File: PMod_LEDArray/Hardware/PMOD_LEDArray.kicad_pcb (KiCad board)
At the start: 2 copper layers, 81.6 x 23 mm, 133 parts, among them J1 Conn_02x06_Odd_Even, U1 GN1640

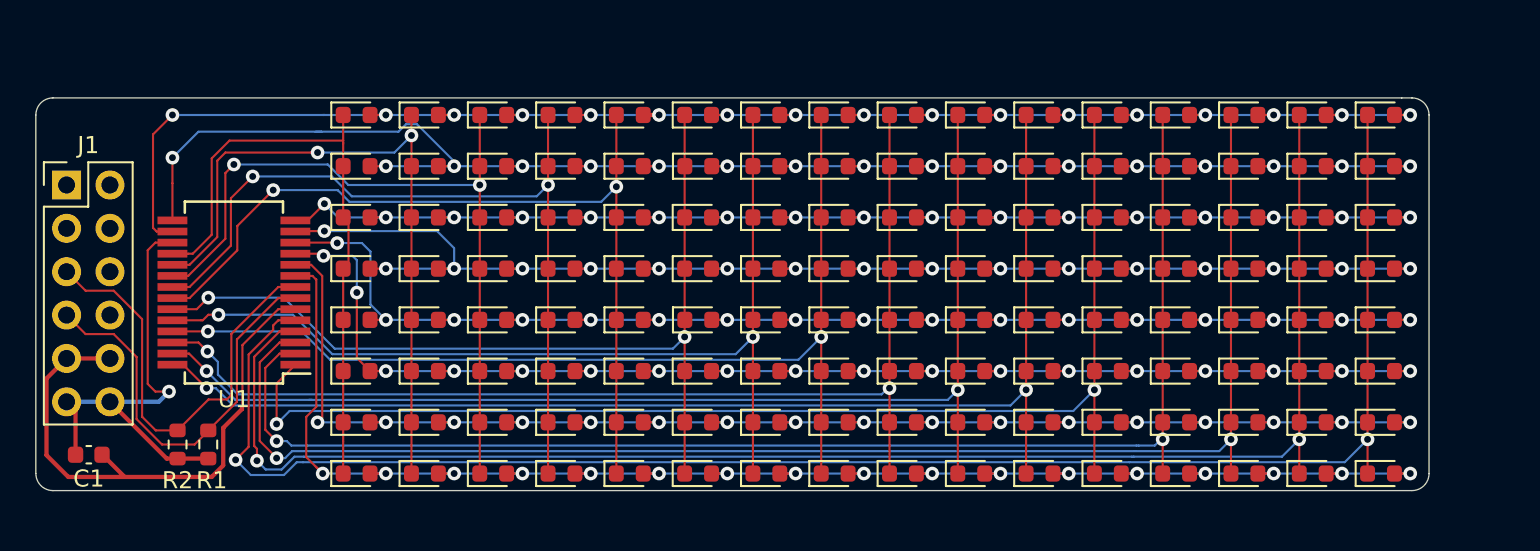
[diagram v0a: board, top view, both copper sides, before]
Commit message: Add mounting holes
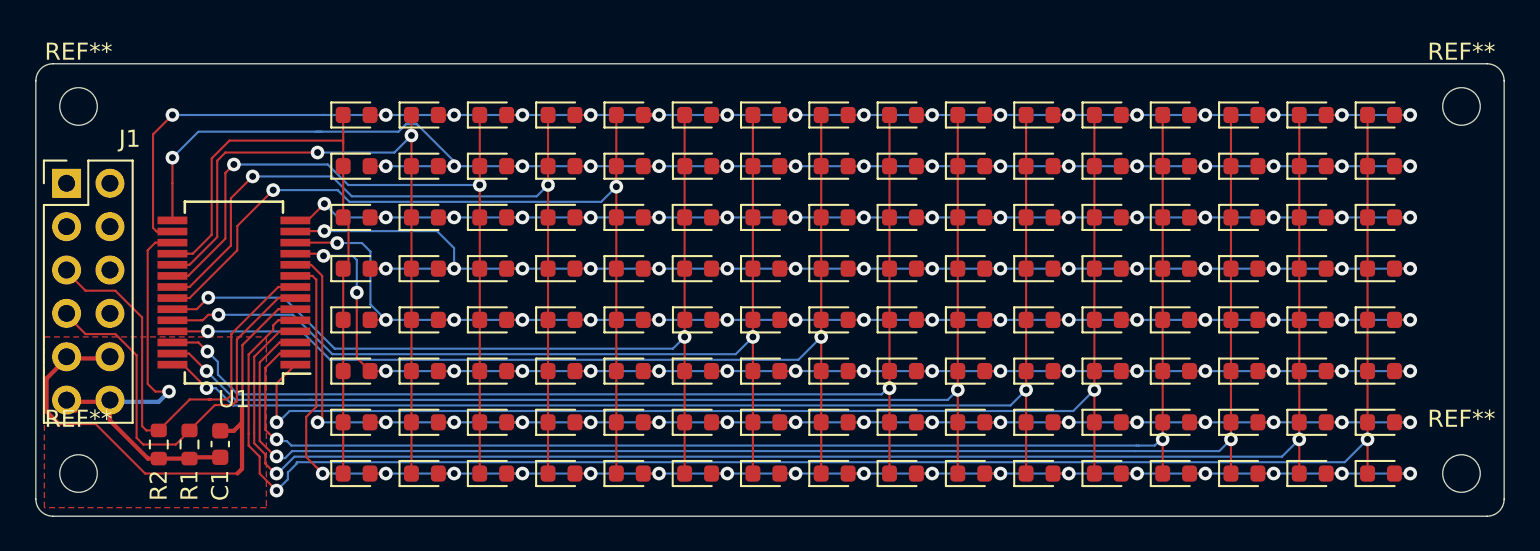
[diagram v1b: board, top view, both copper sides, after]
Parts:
- added REF**: MountingHole_2.2mm_M2, MountingHole:MountingHole_2.2mm_M2, F.Cu at (188.5, 109.0)
- added REF**: MountingHole_2.2mm_M2, MountingHole:MountingHole_2.2mm_M2, F.Cu at (188.5, 87.5)
- added REF**: MountingHole_2.2mm_M2, MountingHole:MountingHole_2.2mm_M2, F.Cu at (107.5, 109.0)
- added REF**: MountingHole_2.2mm_M2, MountingHole:MountingHole_2.2mm_M2, F.Cu at (107.5, 87.5)
- moved C1 7.73 mm to (115.8, 107.3), turned to 90 degrees
- moved R1 1.10 mm to (114.0, 107.3)
- moved R2 1.10 mm to (112.2, 107.3)
- moved J1 0.10 mm to (106.8, 92.0)
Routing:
- net +3V3: track 30.3 -> 26.4 mm
- net GND: track 34.8 -> 32.0 mm
- net DATA: track 24.4 -> 25.1 mm
- net CLK: track 26.2 -> 26.7 mm
- added copper zone on F.Cu, net GND
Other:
- board size 81.6 x 23 mm -> 86 x 26.5 mm
